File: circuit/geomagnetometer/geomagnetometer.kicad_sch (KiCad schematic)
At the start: 20 parts, among them J1 Conn_01x06, U1 RM3100_13156

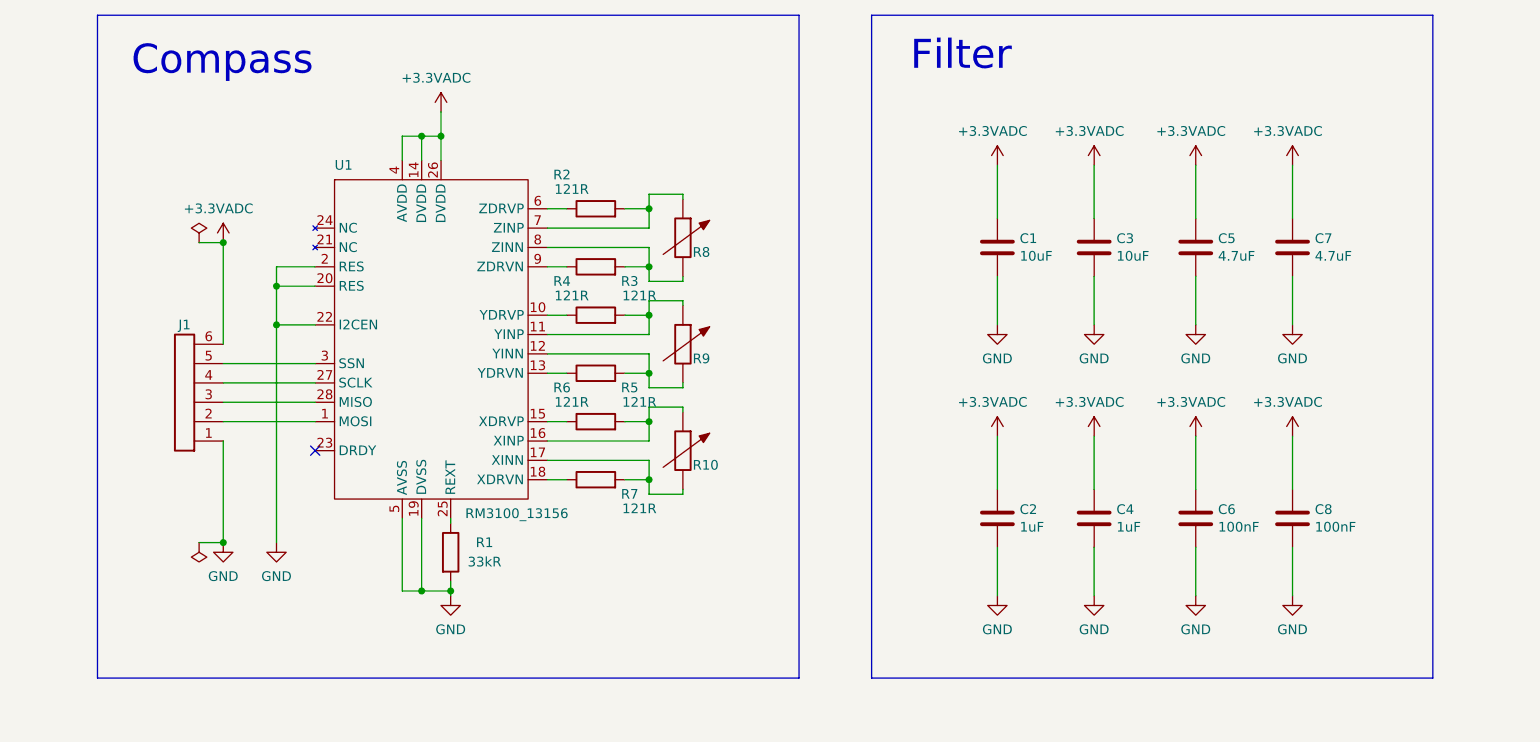
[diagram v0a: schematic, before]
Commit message: Complete the PCB design of the geomagnetometer circuit
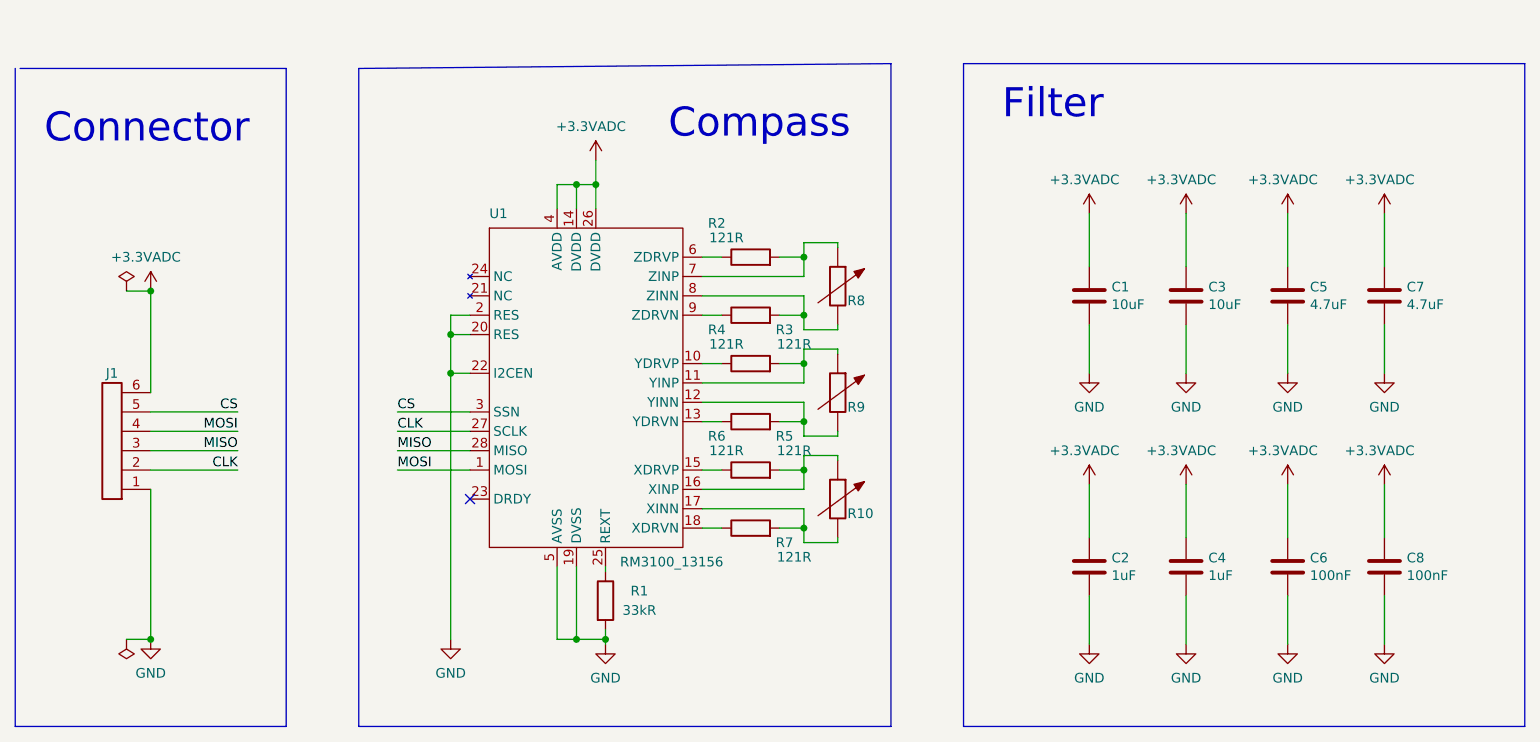
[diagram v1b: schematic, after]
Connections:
- net CLK: now reaches J1.2 (Pin_2)
- net CLK: now also U1.27 (SCLK); no longer U1.1 (MOSI)
- net MOSI: now reaches J1.4 (Pin_4)
- net MOSI: now also U1.1 (MOSI); no longer U1.27 (SCLK)
- net MISO: now reaches J1.3 (Pin_3), U1.28 (MISO)
- net CS: now reaches J1.5 (Pin_5), U1.3 (SSN)
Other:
- note added: "Connector"
- moved on the sheet: C1, C2, C3, C4, C5, C6, C7, C8, J1, R1, R10, R2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
